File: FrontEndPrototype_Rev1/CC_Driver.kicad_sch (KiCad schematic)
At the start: 12 parts, among them U2 ADA4807-2ACP

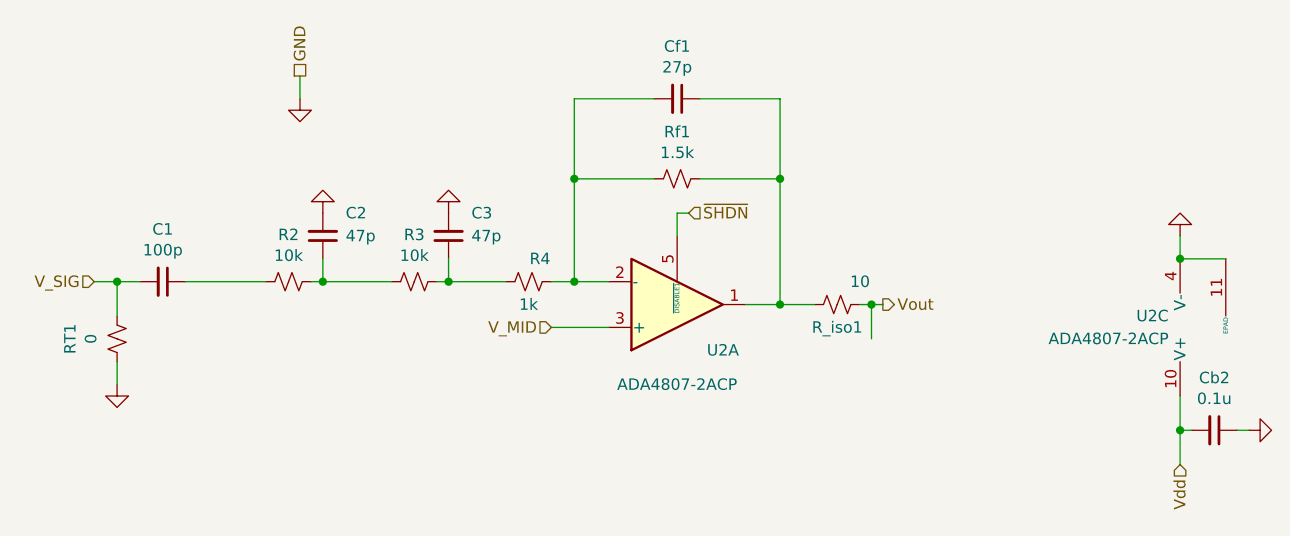
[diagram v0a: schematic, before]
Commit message: First Pass Schematic Fixes for Power Management Board
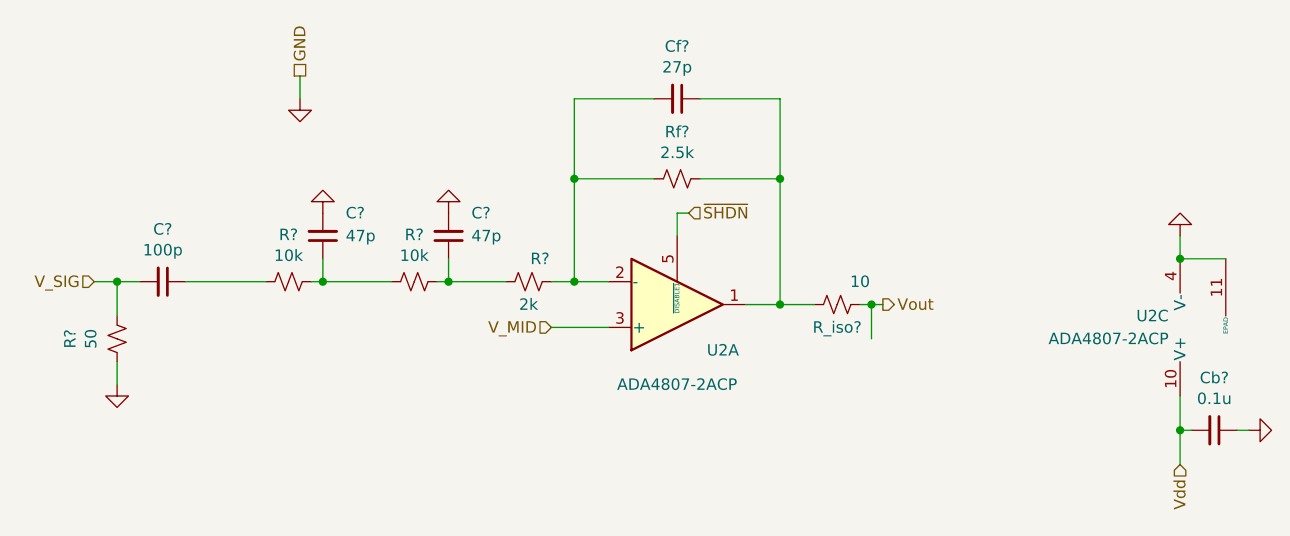
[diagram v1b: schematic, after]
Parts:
- R?: renamed from R4; value 1k -> 2k
- R?: renamed from RT1; value 0 -> 50
- Rf?: renamed from Rf1; value 1.5k -> 2.5k
- renumbered C1 to C?, C2 to C?, C3 to C?, Cb2 to Cb?, Cf1 to Cf?, R2 to R?, R3 to R?, R_iso1 to R_iso?
